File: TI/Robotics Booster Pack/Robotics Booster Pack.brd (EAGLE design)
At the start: 68.6 x 76.2 mm, 100 parts, among them J1 1X2.PTS, U1 TS3A44159.RGT, U11 SCHA4B0400, U13 XBEE-1XBEE-1_LOCK, U14 TPS5450, U15 TPS715XX.DCK, U16 TPS62152.RGT, U3 DRV8800, U4 DRV8800, U5 DRV8800, U6 DRV8800, U7 PCA9557.RGV, U8 MPU-6050, U9 INA220.DGS

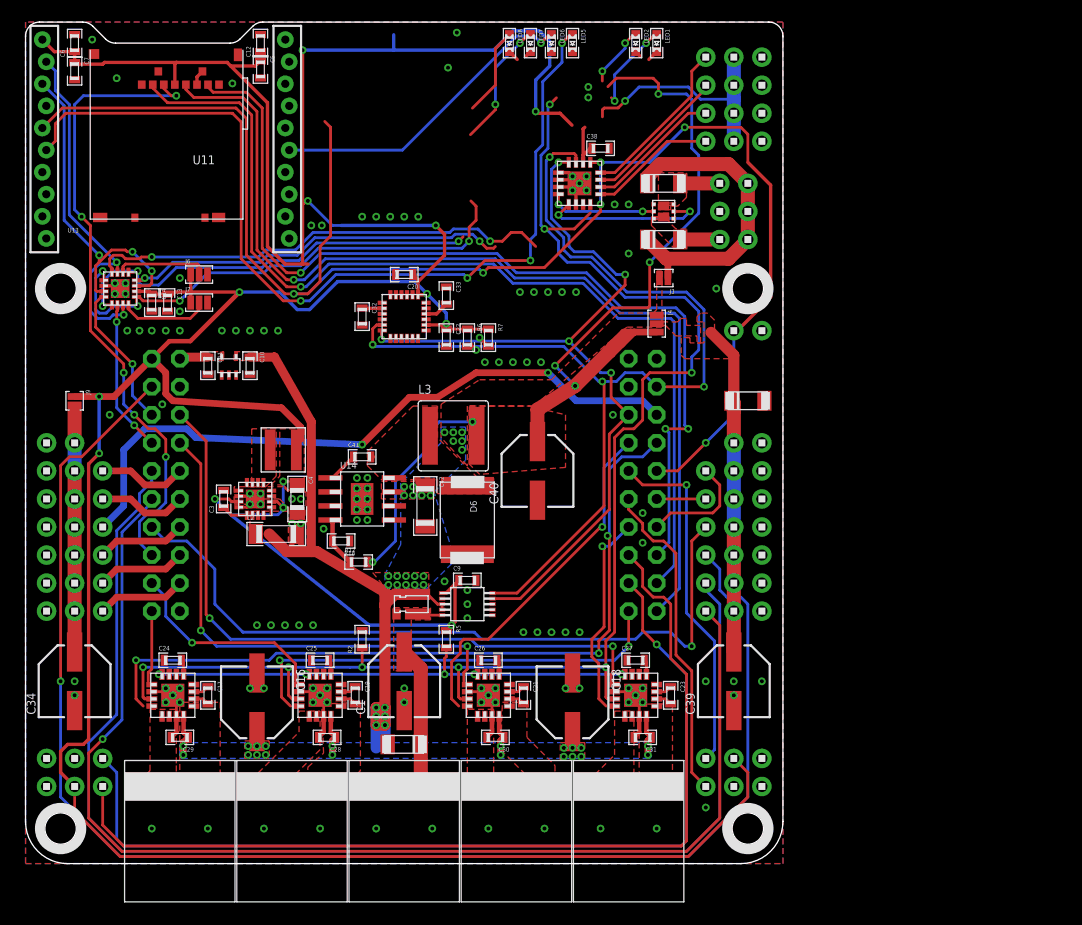
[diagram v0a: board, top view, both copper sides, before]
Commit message: Let the carnage that shall be known as v3 begin!
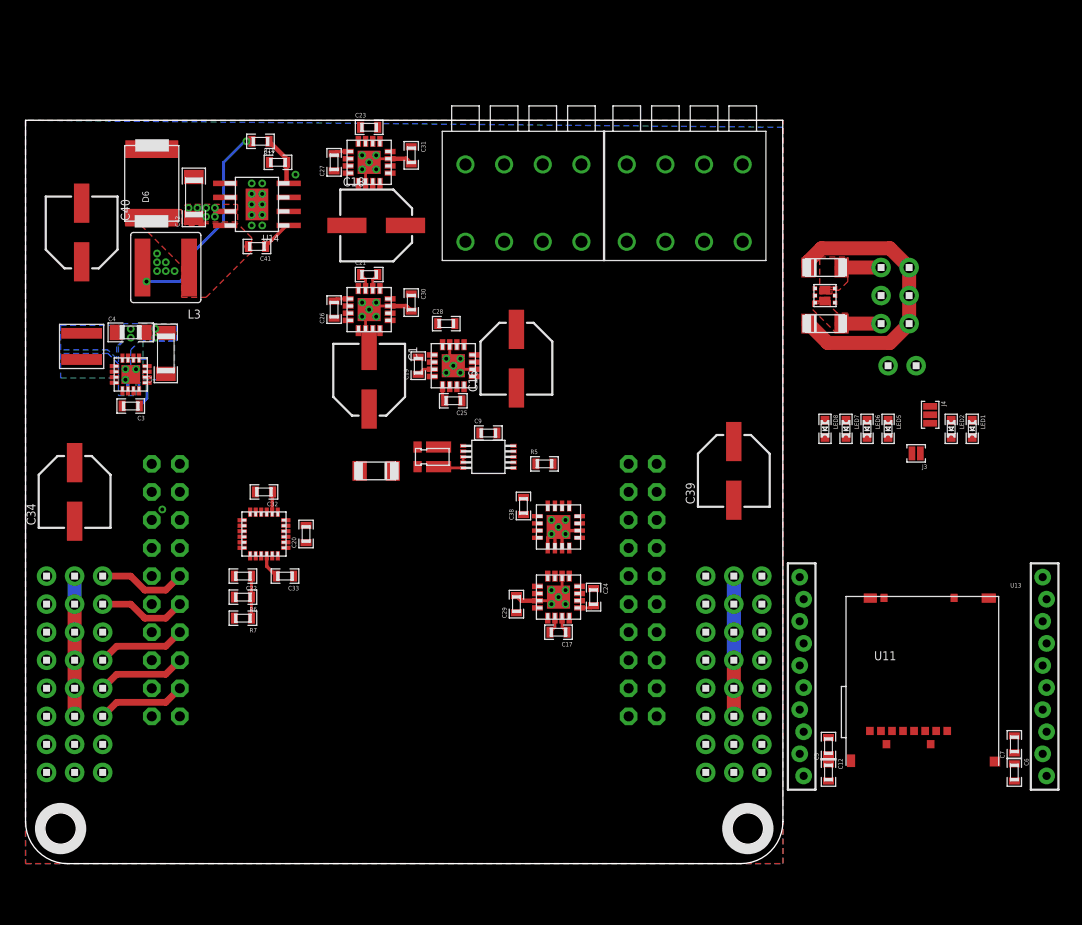
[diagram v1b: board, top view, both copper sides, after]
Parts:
- removed C10, C13: .1uF, standardparts:0603
- removed C11, C14: 1uF, standardparts:0603
- removed D5: CDBMT2100-HF, comchip:SOD-123H
- removed H11, H12: 1X4, headers(.1in):1X4
- removed H17, H18, H19, H20, J1: 1X2.PTS, phoenixcontact:PTS.PLUG
- removed J6, J7: (no value), solderjumper:3.LRG
- removed J9: (no value), solderjumper:2.LRG.PASTE
- removed R2: 10k, standardparts:0603
- removed U$11, U$14: HOLE.4MM, screw_holes:4MM
- removed U1: TS3A44159.RGT, packages(ti):RGT.16
- removed U15: TPS715XX.DCK, packages(ti):DCK
- added H8: 1X4.182440000, weidmuller:1824440000
- H1, H2, H4, H5: value 1X7 -> 1X6; device headers(.1in):1X7 -> headers(.1in):1X6
- H10: value 1X4 -> 1X4.182440000; device headers(.1in):1X4 -> weidmuller:1824440000
- moved C6 107.7 mm to (89.5, 8.26), turned to 270 degrees
- moved C7 104.7 mm to (89.5, 10.8), turned to 90 degrees
- moved U11 84.7 mm to (74.3, 8.89), turned to 0 degrees
- moved C12 83.7 mm to (72.7, 8.26), turned to 270 degrees
- moved C5 80.0 mm to (72.7, 10.6), turned to 90 degrees
- moved U13 73.6 mm to (81.3, 27.9), turned to 180 degrees
- moved C23 58.2 mm to (31.1, 66.7), turned to 0 degrees
- moved C31 56.7 mm to (34.9, 64.1), turned to 270 degrees
- moved U4 54.0 mm to (31.1, 63.5), turned to 90 degrees
- moved C27 52.7 mm to (27.9, 63.5), turned to 90 degrees
- moved C18 46.7 mm to (31.8, 57.8), turned to 0 degrees
- moved C40 46.6 mm to (5.08, 57.1), turned to 270 degrees
- moved LED1 45.1 mm to (85.7, 39.4)
- moved LED2 45.1 mm to (83.8, 39.4)
- moved LED5 45.1 mm to (78.1, 39.4)
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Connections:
- removed net BT.CONNECT: LED8.P$1
- removed net BT.RXI: U1.13, U1.5
- removed net BT.STATUS: LED7.P$1
- removed net BT.TXO: U1.1, U1.9
- removed net IO0: H12.1, U7.12
- removed net IO1: H12.2, U7.11
- removed net IO2: H12.3, U7.10
- removed net IO3: H12.4, U7.9
- removed net M.EN: R2.1, U3.3, U4.3, U5.3, U6.3
- removed net N$2: J6.2, U1.2
- removed net N$3: J7.2, U1.12
- removed net UART0.RXI: U1.4
- removed net UART0.TXO: U1.16
- removed net VBUS: C11.1, U$8.VBUS, U15.5
- new net IMU.INT: U7.5, U8.12
- new net M0.EN: U5.3, U7.9
- new net M1.EN: U6.3, U7.10
- new net M2.EN: U3.3, U7.11
- new net M3.EN: U4.3, U7.12
- new net XBEE.CONNECTED: U13.17, U7.4
- net 3.3V: no longer C13.1, C14.1, H11.1, H11.2, H11.3, H11.4, J6.1, J7.1, J9.1, U1.14
- net 5.0V: now also U$8.VBUS
- net FET0.G: now also U7.7; no longer U7.4
- net FET1.G: now also U7.8; no longer U7.5
- net GND: no longer C10.2, C11.2, C13.2, C14.2, D5.2, H1.7, H10.1, H10.2, H10.3, H10.4, H4.7, J1.2, J6.3, J7.3, R2.2, U1.6, U1.PAD, U15.2
- net M0+: now also H8.1@1, H8.1@2; no longer H17.1
- net M0-: now also H8.2@1, H8.2@2; no longer H17.2
- net M0.DIR: now also U$8.PC4; no longer U$8.PF0
- net M1+: now also H8.3@1, H8.3@2; no longer H18.1
- net M1-: now also H8.4@1, H8.4@2; no longer H18.2
- net M1.DIR: now also U$8.PC7; no longer U$8.PF4
- net M2+: now also H10.1@1, H10.1@2; no longer H19.1
- net M2-: now also H10.2@1, H10.2@2; no longer H19.2
- net M2.DIR: now also U$8.PF0; no longer U$8.PC4
- net M3+: now also H10.3@1, H10.3@2; no longer H20.1
- net M3-: now also H10.4@1, H10.4@2; no longer H20.2
- net M3.DIR: now also U$8.PF4; no longer U$8.PC7
- net N$22: no longer J1.1
- net N$4: no longer H5.7, J9.2
- net UART1.RXI: no longer U1.8
- net UART1.TXO: no longer U1.10
- net VBAT: no longer C10.1, U15.4
- net VSERVO: no longer D5.1, H2.7
- net XBEE.RXI: no longer U1.11, U1.3
- net XBEE.TXO: no longer U1.15, U1.7
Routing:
- net 3.3V: track 380.3 -> 3.81 mm, vias 14 -> 0
- net !RST: track 144.0 -> 0.00 mm, vias 6 -> 0
- net SVRO3: track 132.1 -> 0.00 mm, vias 1 -> 0
- net M.EN: track 131.6 -> 0.00 mm, vias 8 -> 0
- net SVRO4: track 115.2 -> 0.00 mm
- net SVRO5: track 110.2 -> 0.00 mm, vias 1 -> 0
- net I2C.SCL: track 95.1 -> 0.00 mm, vias 5 -> 0
- net SPI.SCLK: track 90.0 -> 0.00 mm, vias 1 -> 0
- net SPI.!CS: track 89.6 -> 0.00 mm, vias 1 -> 0
- net QEI0.A: track 85.9 -> 0.00 mm
- net QEI0.B: track 85.4 -> 0.00 mm, vias 1 -> 0
- net SPI.MISO: track 85.3 -> 0.00 mm, vias 3 -> 0
- net XBEE.RSSI: track 84.3 -> 0.00 mm, vias 4 -> 0
- net VBAT: track 81.8 -> 1.20 mm, vias 48 -> 12
- net I2C.SDA: track 75.9 -> 0.00 mm, vias 6 -> 0
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- added copper zone on layer 16, net 3.3V
- added copper zone on layer 16, net N$1
- removed copper zone on layer 1, net 3.3V
- removed copper zone on layer 1, net 5.0V
- removed copper zone on layer 1, net M0+
- removed copper zone on layer 1, net M0-
- removed copper zone on layer 1, net M1+
- removed copper zone on layer 1, net M1-
- removed copper zone on layer 1, net M2+
- removed copper zone on layer 1, net M2-
- removed copper zone on layer 1, net M3+
- removed copper zone on layer 1, net M3-
- removed copper zone on layer 1, net N$1
- removed copper zone on layer 1, net N$16
- removed copper zone on layer 1, net N$22
- removed copper zone on layer 1, net VBUS
- removed copper zone on layer 1, net VSERVO
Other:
- board size 68.6 x 76.2 mm -> 68.6 x 67.3 mm
- board text removed: "3.3v"
- board text removed: "5V"
- board text removed: "5v"
- board text removed: "ADC"
- board text removed: "Associate"
- board text removed: "BT"
- board text removed: "Connect"
- board text removed: "ENC 0"
- board text removed: "ENC 1"
- board text removed: "GPIO"
- board text removed: "M0"
- board text removed: "M1"
- board text removed: "M2"
- board text removed: "M3"
- board text removed: "Motors ON"
- board text removed: "RSSI"
- board text removed: "SERVO"
- board text removed: "Servos ON"
- board text removed: "Status"
- board text removed: "UART0"
- board text removed: "UART1"
- board text removed: "VBAT"
- board text removed: "VSRVO"
- board text removed: "VSVRO"
- board text removed: "XBee"
